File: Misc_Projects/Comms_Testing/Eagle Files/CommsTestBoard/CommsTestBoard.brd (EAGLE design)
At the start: 76.2 x 100 mm, 12 parts, among them J1 1985205, J2 1985205

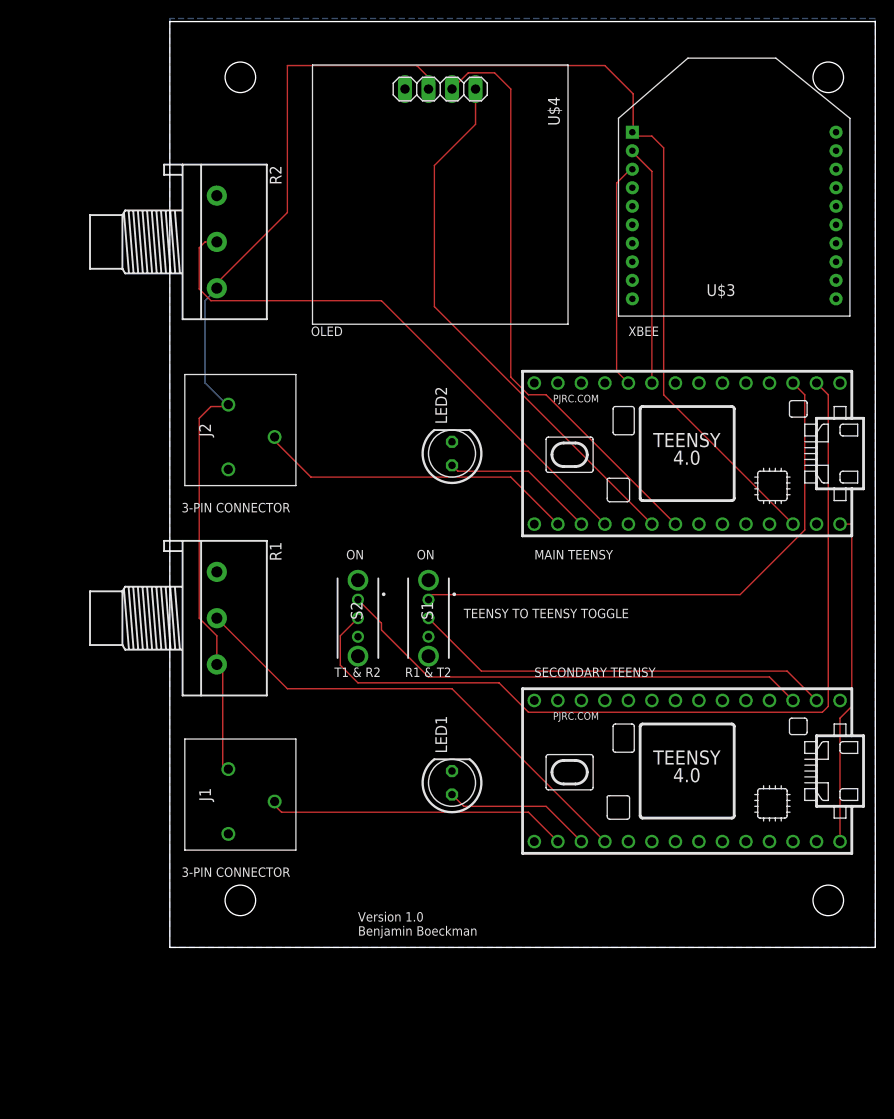
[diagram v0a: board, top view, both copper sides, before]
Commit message: Updated comms testing board
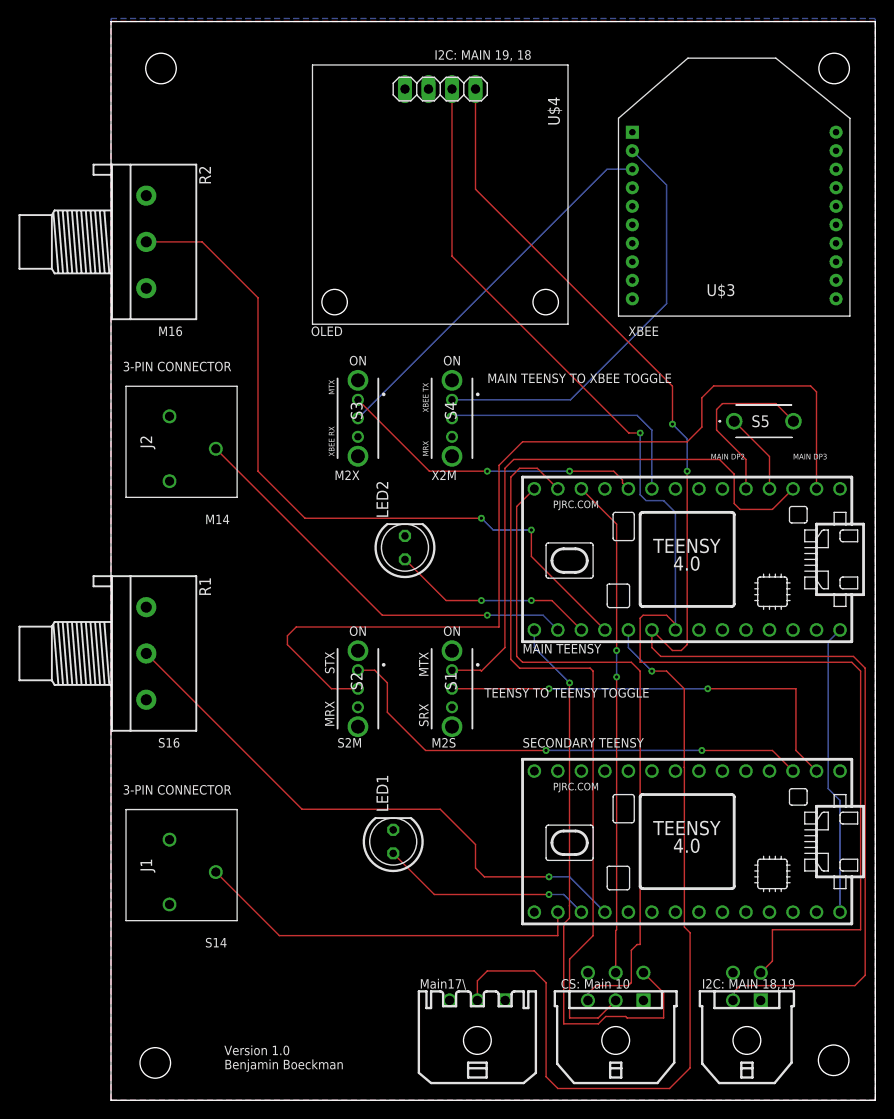
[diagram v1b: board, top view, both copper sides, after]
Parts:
- added S3, S4: SWITCH_SLIDE_OS102011MS2QN1, GTOR - Active Components:OS102011MA1QN1
- added S5: PTS636_SL50_LFS, GTOR - Active Components:PTS636SL50LFS
- added X1: (no value), GTOR - Microfit Connector:43045-0400
- added X2: (no value), GTOR - Microfit Connector:43650-0300
- added X3: (no value), GTOR - Microfit Connector:43045-0600
- moved U$2 11.4 mm to (55.9, 41.9)
- moved LED2 11.4 mm to (25.4, 43.2)
- moved J1 9.92 mm to (1.27, 8.89)
- moved LED1 8.98 mm to (24.1, 11.4)
- moved R1 8.52 mm to (-2.54, 31.8)
- moved S1 8.03 mm to (30.5, 27.9)
- moved S2 7.62 mm to (20.3, 27.9)
- moved U$1 7.62 mm to (55.9, 11.4)
- moved R2 7.62 mm to (-2.54, 76.2)
- moved J2 6.48 mm to (1.27, 54.6)
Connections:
- new net A1: U$2.17/A3, X2.P$2
- new net CS: U$2.10/CS, X3.P$5
- new net DP: S5.1, U$2.2
- new net DP2: S5.2, U$2.3/CANTX
- new net MISO: U$2.12/MISO, X3.P$3
- new net MOSI: U$2.11/MOSI, X3.P$2
- new net R4: S4.2, U$2.7
- new net SCK: U$2.13/SCK, X3.P$4
- new net T4: S4.1, U$3.2
- net 3V3: now also X1.P$1, X2.P$1, X3.P$1
- net GND: now also X1.P$4, X2.P$3, X3.P$6
- net R3: now also S3.2; no longer U$2.8
- net SCL: now also X1.P$3
- net SDA: now also X1.P$2
- net T3: now also S3.1, U$2.8; no longer U$2.7, U$3.2
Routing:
- net 3V3: track 181.9 -> 0.00 mm
- net SDA: track 58.6 -> 149.4 mm, vias 0 -> 2
- net A1: track 0.00 -> 88.7 mm, vias 0 -> 1
- net SCL: track 63.3 -> 146.8 mm, vias 0 -> 1
- net MOSI: track 0.00 -> 79.8 mm
- net MISO: track 0.00 -> 73.0 mm
- net SCK: track 0.00 -> 61.4 mm, vias 0 -> 1
- net CS: track 0.00 -> 53.9 mm, vias 0 -> 2
- net T4: track 0.00 -> 45.5 mm
- net R4: track 0.00 -> 28.7 mm
- net DP2: track 0.00 -> 19.2 mm
- net P2: track 60.9 -> 79.5 mm, vias 0 -> 2
- net R3: track 24.4 -> 40.8 mm
- net P1: track 51.9 -> 62.6 mm, vias 0 -> 1
- net C2: track 34.7 -> 45.0 mm, vias 0 -> 1
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- added copper zone on layer 1, net 3V3
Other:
- board size 76.2 x 100 mm -> 82.5 x 116.5 mm
- board text added: "CS: Main 10"
- board text added: "I2C: MAIN 18,19"
- board text added: "I2C: MAIN 19, 18"
- board text added: "M14"
- board text added: "M16"
- board text added: "M2S"
- board text added: "M2X"
- board text added: "MAIN DP2"
- board text added: "MAIN DP3"
- board text added: "MAIN TEENSY TO XBEE TOGGLE"
- board text added: "MRX"
- board text added: "MTX"
- board text added: "Main17\"
- board text added: "S14"
- board text added: "S16"
- board text added: "S2M"
- board text added: "SRX"
- board text added: "STX"
- board text added: "X2M"
- board text added: "XBEE RX"
- board text added: "XBEE TX"
- board text removed: "R1 & T2"
- board text removed: "T1 & R2"
